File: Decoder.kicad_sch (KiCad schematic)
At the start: 10 parts, among them P1 IO_ADDR, P17 RTC_IO_ADDR, U2 74LS14, U21 74LS682N, U33 74LS10, U39 74LS04, U57 74LS682N, U58 74LS138, U68 74LS138, U7 74LS32

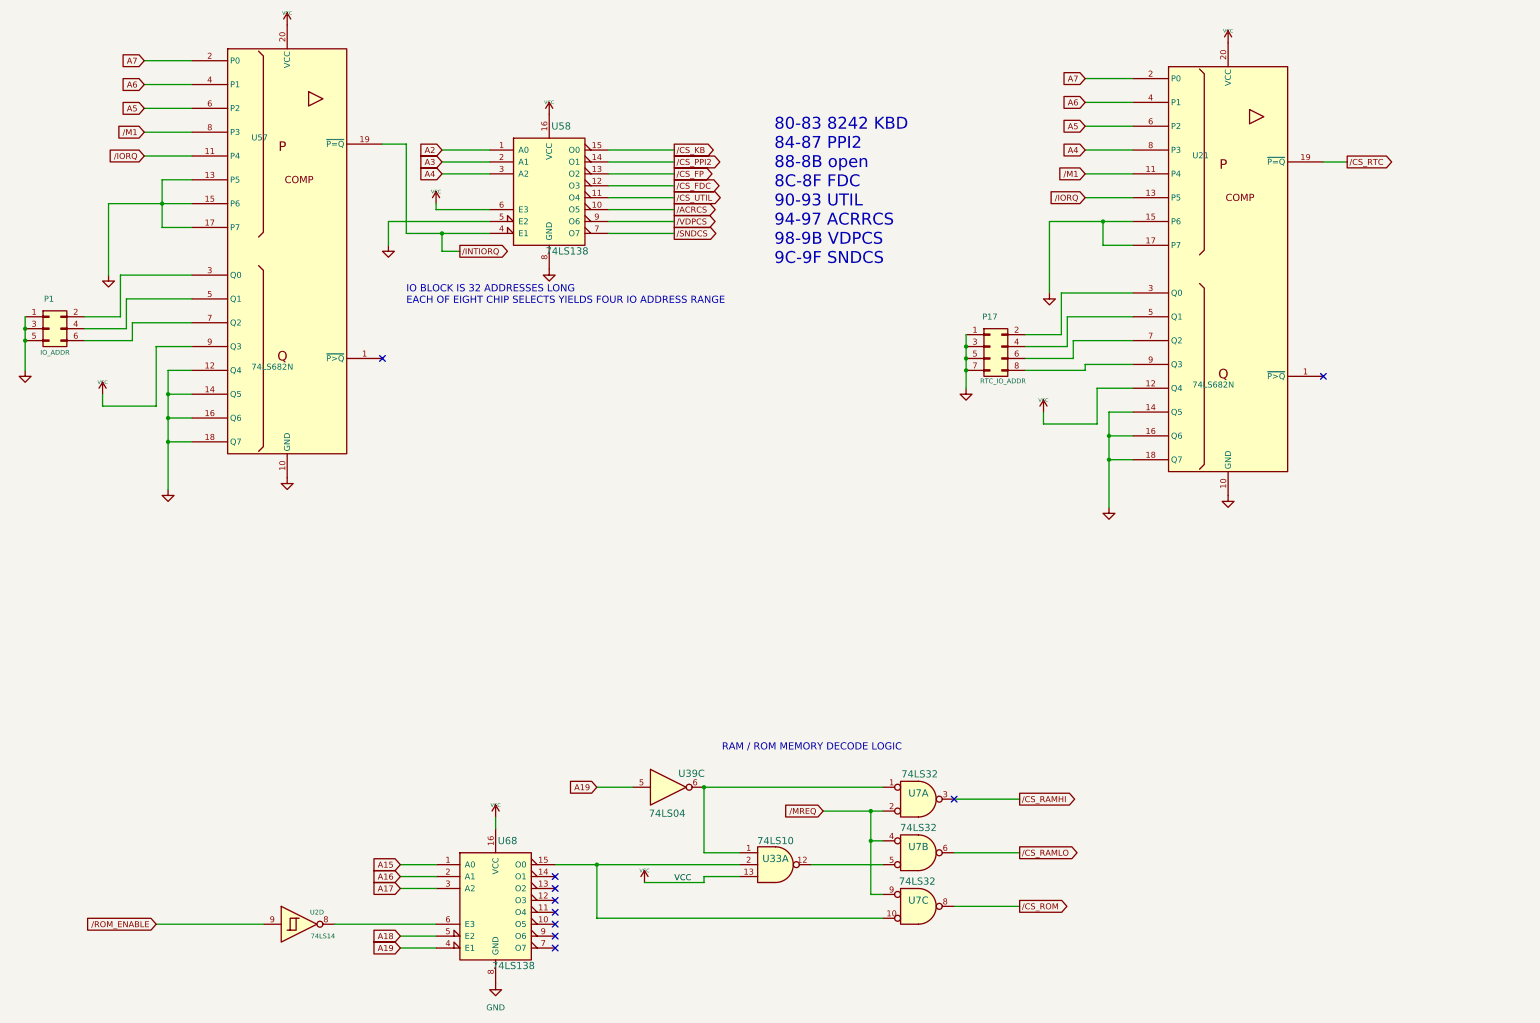
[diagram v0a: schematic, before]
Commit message: V1
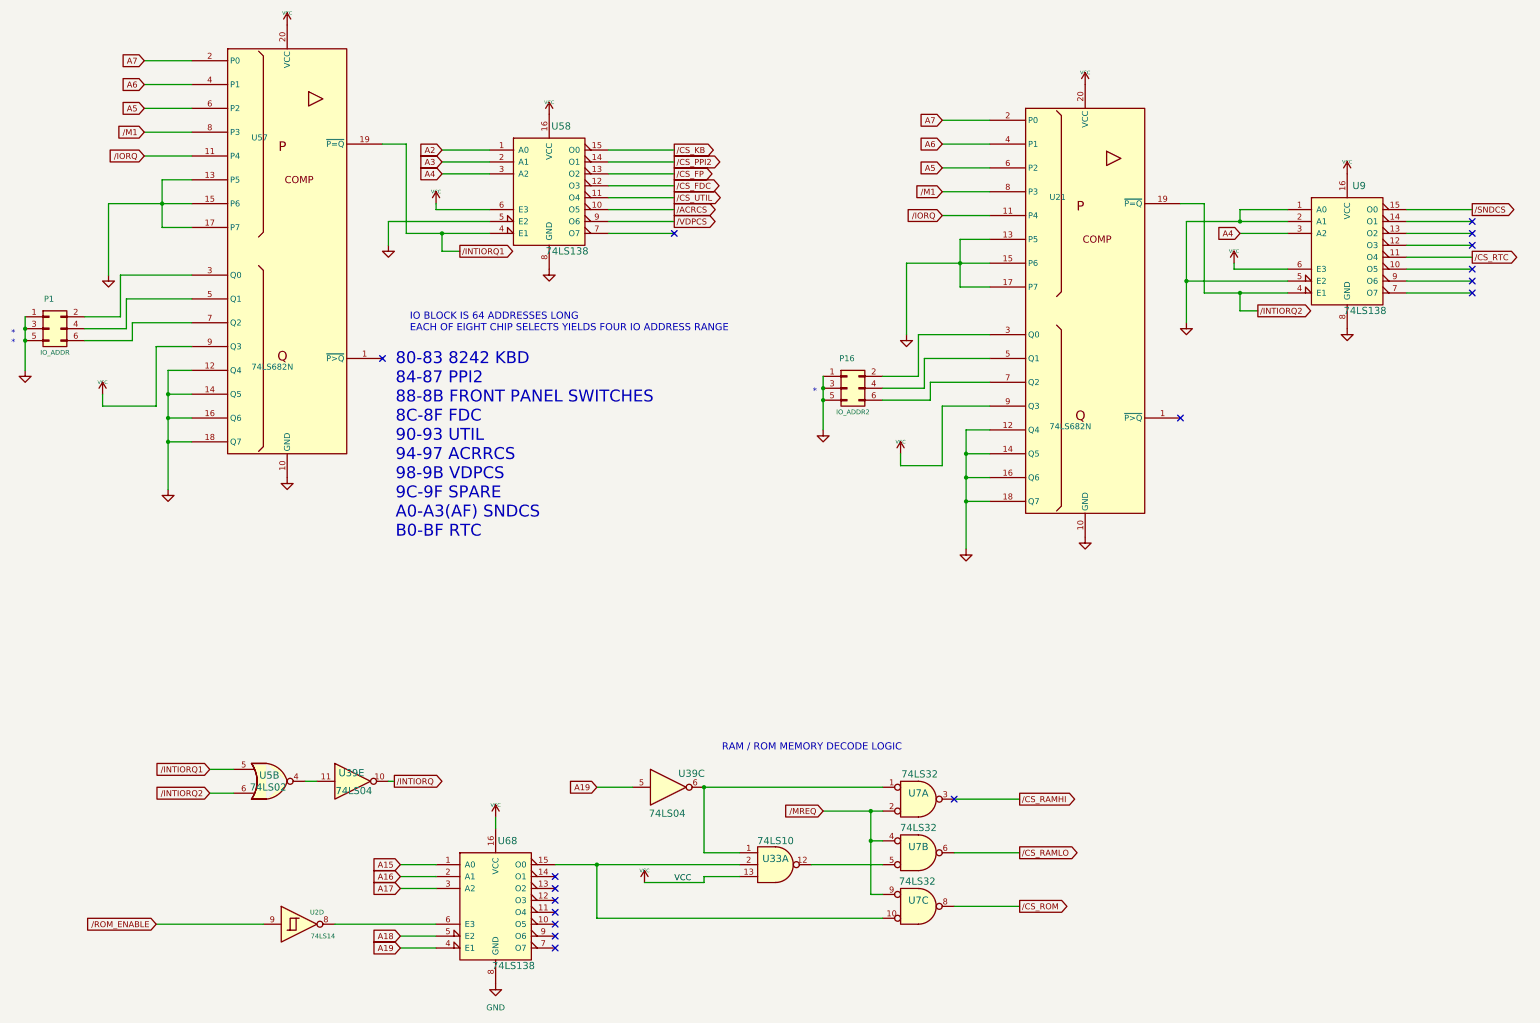
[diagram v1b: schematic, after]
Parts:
- removed P17: RTC_IO_ADDR, Custom:STD_DDW_PINHEAD_V_2x04, symbol Connector_Generic:Conn_02x04_Odd_Even
- added P16: IO_ADDR2, Custom:STD_DDW_PinHeader_2x03, symbol Connector_Generic:Conn_02x03_Odd_Even
- added unit 5 of U39
- added U5: 74LS02, Custom:STD_DDW_DIP14, symbol 74xx:74LS02
- added U9: 74LS138, Custom:STD_DDW_DIP16, symbol 74xx:74LS138
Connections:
- net A4: now also U9.3 (A2); no longer U21.8 (P3)
- net GND: now also U21.12 (Q4), U21.13 (P5), P16.1 (Pin_1), P16.3 (Pin_3), P16.5 (Pin_5), U9.1 (A0), U9.2 (A1), U9.5 (E2), U9.8 (GND)
- net VCC: now also U21.9 (Q3), U9.16 (VCC), U9.6 (E3); no longer U21.12 (Q4)
- net /CS_RTC: now also U9.11 (O4); no longer U21.19 (~{P=Q})
- net /INTIORQ: now also U39.10; no longer U57.19 (~{P=Q}), U58.4 (E1)
- net /IORQ: now also U21.11 (P4); no longer U21.13 (P5)
- net /M1: now also U21.8 (P3); no longer U21.11 (P4)
- net /SNDCS: now also U9.15 (O0); no longer U58.7 (O7)
- net at U21.3 (Q0): now also P16.2 (Pin_2)
- net at U21.5 (Q1): now also P16.4 (Pin_4)
- net at U21.7 (Q2): now also P16.6 (Pin_6)
- new net: U39.11, U5.4
- new net /INTIORQ1: U5.5, U57.19 (~{P=Q}), U58.4 (E1)
- new net /INTIORQ2: U21.19 (~{P=Q}), U5.6, U9.4 (E1)
- no-connect marks 10 -> 17
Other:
- note added: "*"
- note added: "* *"
- note added: "80-83 8242 KBD 84-87 PPI2 88-8B FRONT PANEL SWITCHES 8C-8F FDC 90-93 UTIL 94-97 ACRRCS 98-9B VDPCS 9C-9F SPARE A0-A3(AF) SNDCS B0-BF RTC"
- note added: "IO BLOCK IS 64 ADDRESSES LONG EACH OF EIGHT CHIP SELECTS YIELDS FOUR IO ADDRESS RANGE"
- note removed: "80-83 8242 KBD 84-87 PPI2 88-8B open 8C-8F FDC 90-93 UTIL 94-97 ACRRCS 98-9B VDPCS 9C-9F SNDCS"
- note removed: "IO BLOCK IS 32 ADDRESSES LONG EACH OF EIGHT CHIP SELECTS YIELDS FOUR IO ADDRESS RANGE"
- moved on the sheet: U21
